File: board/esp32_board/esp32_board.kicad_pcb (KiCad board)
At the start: 2 copper layers, 95.5 x 110 mm, 11 parts, among them J1 Screw_Terminal_01x19, J2 Screw_Terminal_01x19, J3 Conn_01x19_Socket, J4 Conn_01x19_Pin, J5 Conn_01x19_Socket, J6 Conn_01x19_Pin, U1 ESP32-DevKitC

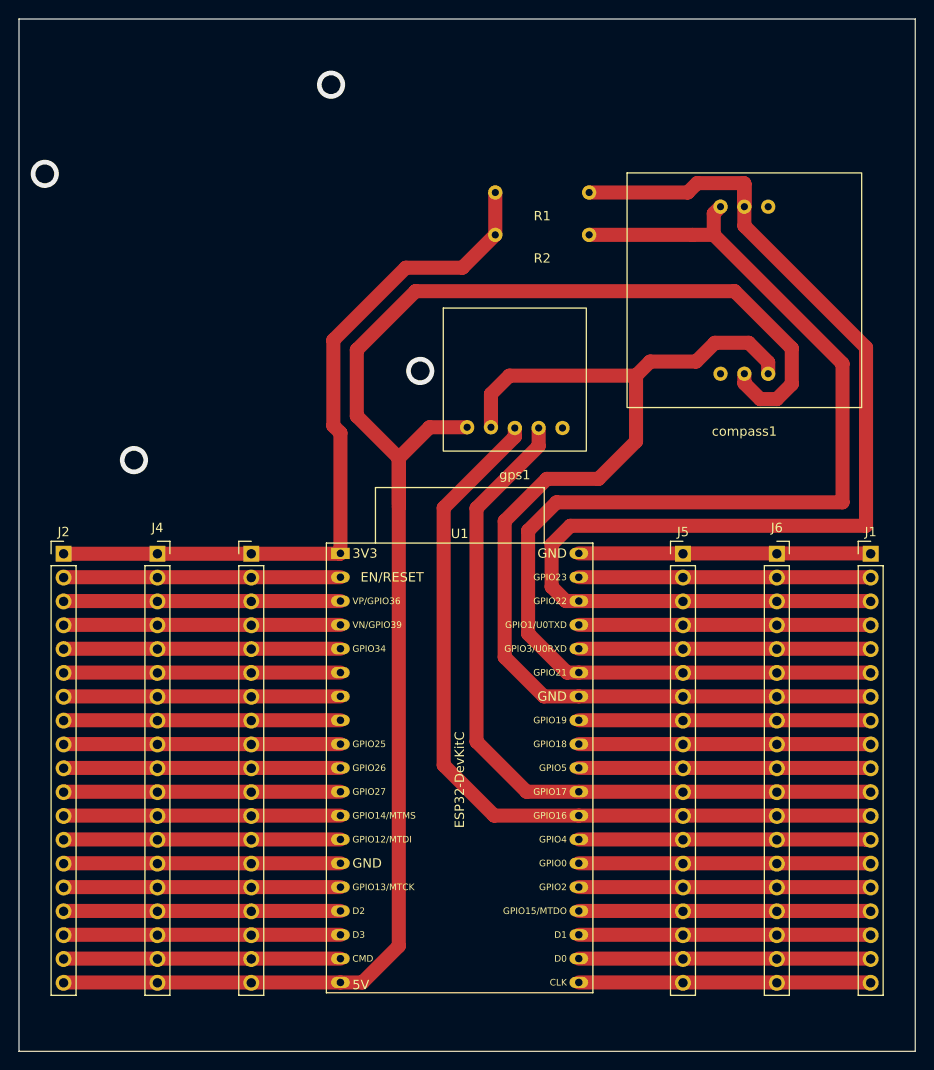
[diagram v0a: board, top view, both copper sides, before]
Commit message: feat: Final board version and updated docs
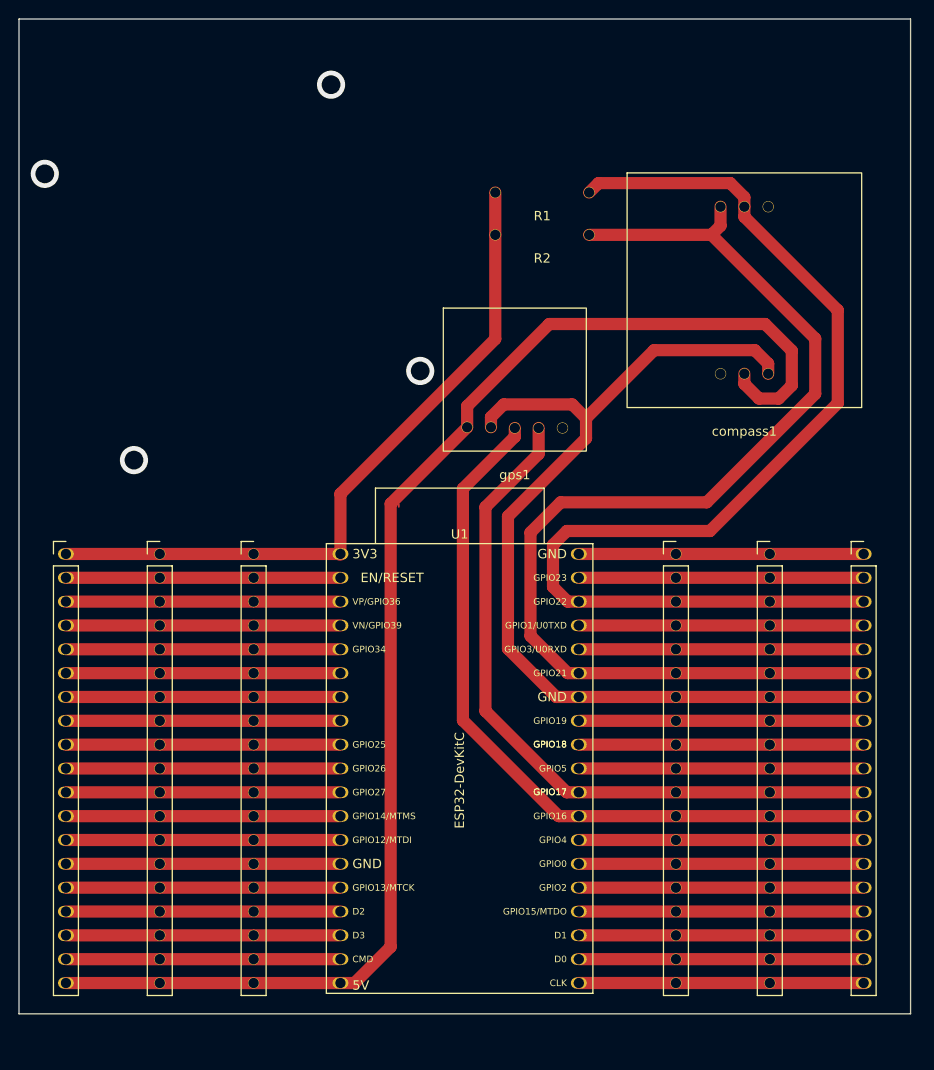
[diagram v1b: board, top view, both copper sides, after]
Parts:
- J1, J2, J3, J5: footprint Connector_PinHeader_2.54mm:PinHeader_1x19_P2.54mm_Vertical -> slon_modules:PinHeader_1x19_P2.54mm_Vertical
- J4, J6: footprint Connector_PinSocket_2.54mm:PinSocket_1x19_P2.54mm_Vertical -> slon_modules:PinHeader_1x19_P2.54mm_Vertical
- moved J4 10.3 mm to (125.2, 92.5)
- moved J3 9.75 mm to (115.2, 92.5)
- moved J1 0.75 mm to (190.2, 92.5)
- moved J5 0.75 mm to (170.2, 92.5)
- moved J6 0.75 mm to (180.2, 92.5)
- moved J2 0.25 mm to (105.2, 92.5)
- moved U1 0.06 mm to (134.5, 92.5)
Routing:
- net V5: track 179.3 -> 147.9 mm
- net 22: track 134.7 -> 118.5 mm
- net GND: track 177.8 -> 164.1 mm
- net 21: track 134.7 -> 122.6 mm
- net 16: track 86.8 -> 80.4 mm
- net 3V3: track 79.0 -> 74.7 mm
- net 17: track 80.4 -> 76.4 mm
- net 15: track 31.1 -> 30.3 mm
- net RX: track 31.1 -> 30.3 mm
- net 5: track 31.1 -> 30.3 mm
- net 19: track 31.1 -> 30.3 mm
- net 0: track 31.1 -> 30.3 mm
- net TX: track 31.1 -> 30.3 mm
- net SD1: track 31.1 -> 30.3 mm
- net SD0: track 31.1 -> 30.4 mm
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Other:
- board size 95.5 x 110 mm -> 95 x 106 mm
- board text added: "GPIO17"
- board text added: "GPIO18"
